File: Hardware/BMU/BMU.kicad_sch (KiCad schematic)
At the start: 5 parts, among them J1 IN/GND, J2 COM, J3 I2C, J4 CAN, J5 SHUNT

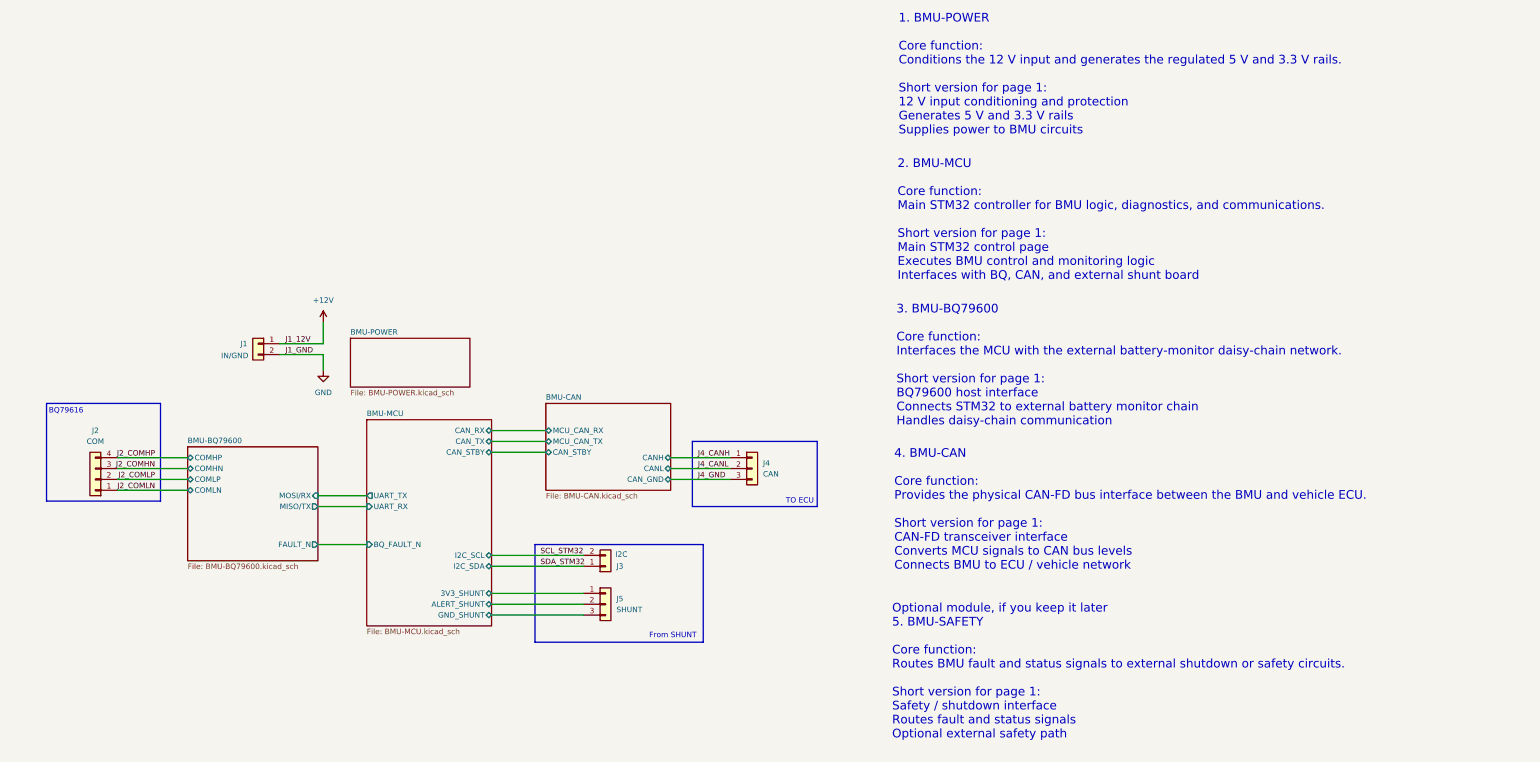
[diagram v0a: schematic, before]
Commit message: add iso
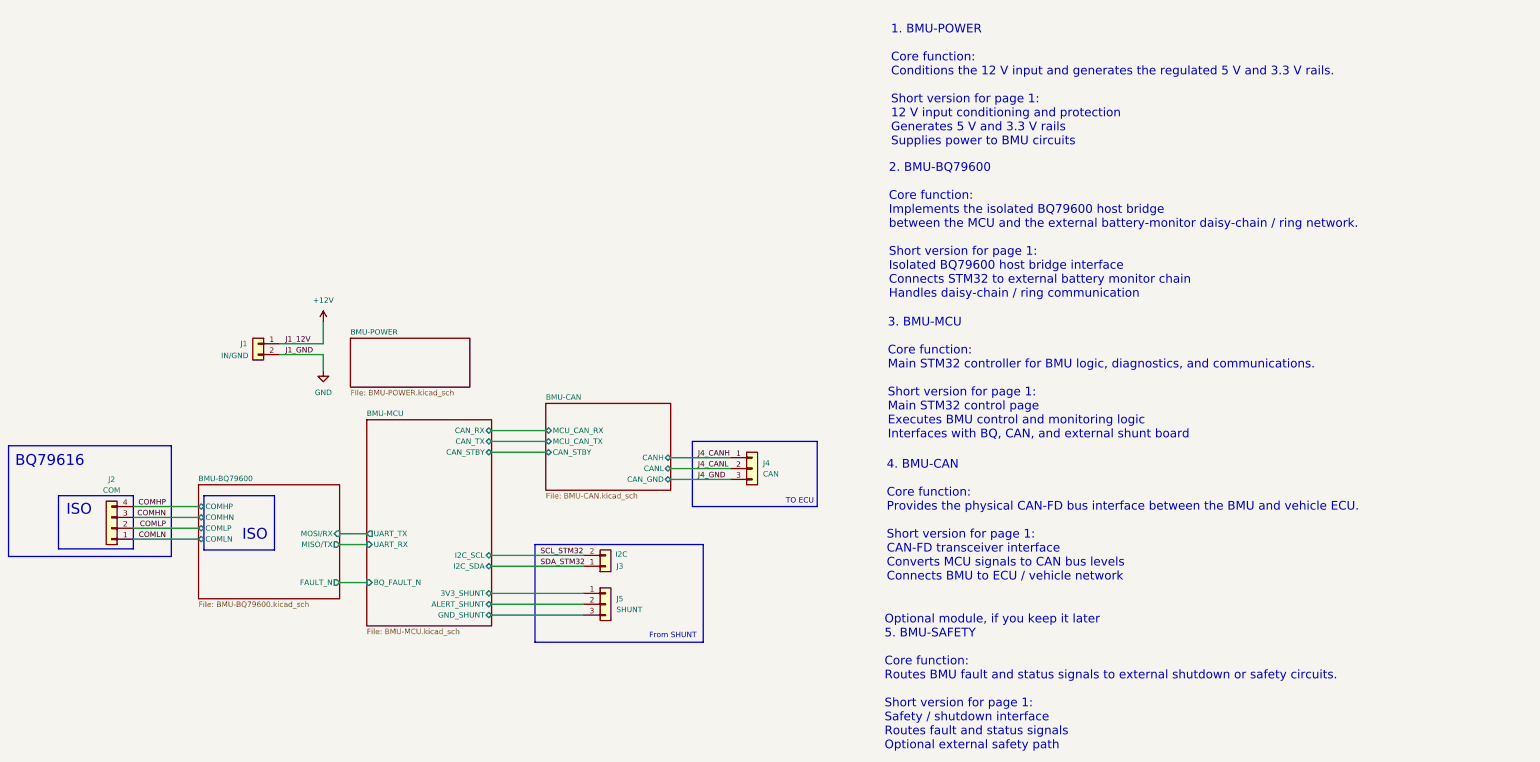
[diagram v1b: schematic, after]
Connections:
- net J2_COMHN renamed COMHN
- net J2_COMHP renamed COMHP
- net J2_COMLN renamed COMLN
- net J2_COMLP renamed COMLP
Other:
- note added: "2. BMU-BQ79600 Core function: Implements the isolated BQ79600 host bridge between the MCU and the external battery-monitor daisy-chain / ring network. Short version for page 1: Isolated BQ79600 host bridge interface Connects STM32 to external battery monitor chain Handles daisy-chain / ring communication"
- note added: "3. BMU-MCU Core function: Main STM32 controller for BMU logic, diagnostics, and communications. Short version for page 1: Main STM32 control page Executes BMU control and monitoring logic Interfaces with BQ, CAN, and external shunt board"
- note added: "ISO"
- note removed: "2. BMU-MCU Core function: Main STM32 controller for BMU logic, diagnostics, and communications. Short version for page 1: Main STM32 control page Executes BMU control and monitoring logic Interfaces with BQ, CAN, and external shunt board"
- note removed: "3. BMU-BQ79600 Core function: Interfaces the MCU with the external battery-monitor daisy-chain network. Short version for page 1: BQ79600 host interface Connects STM32 to external battery monitor chain Handles daisy-chain communication"
